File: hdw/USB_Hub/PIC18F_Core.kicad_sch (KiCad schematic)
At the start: 3 parts

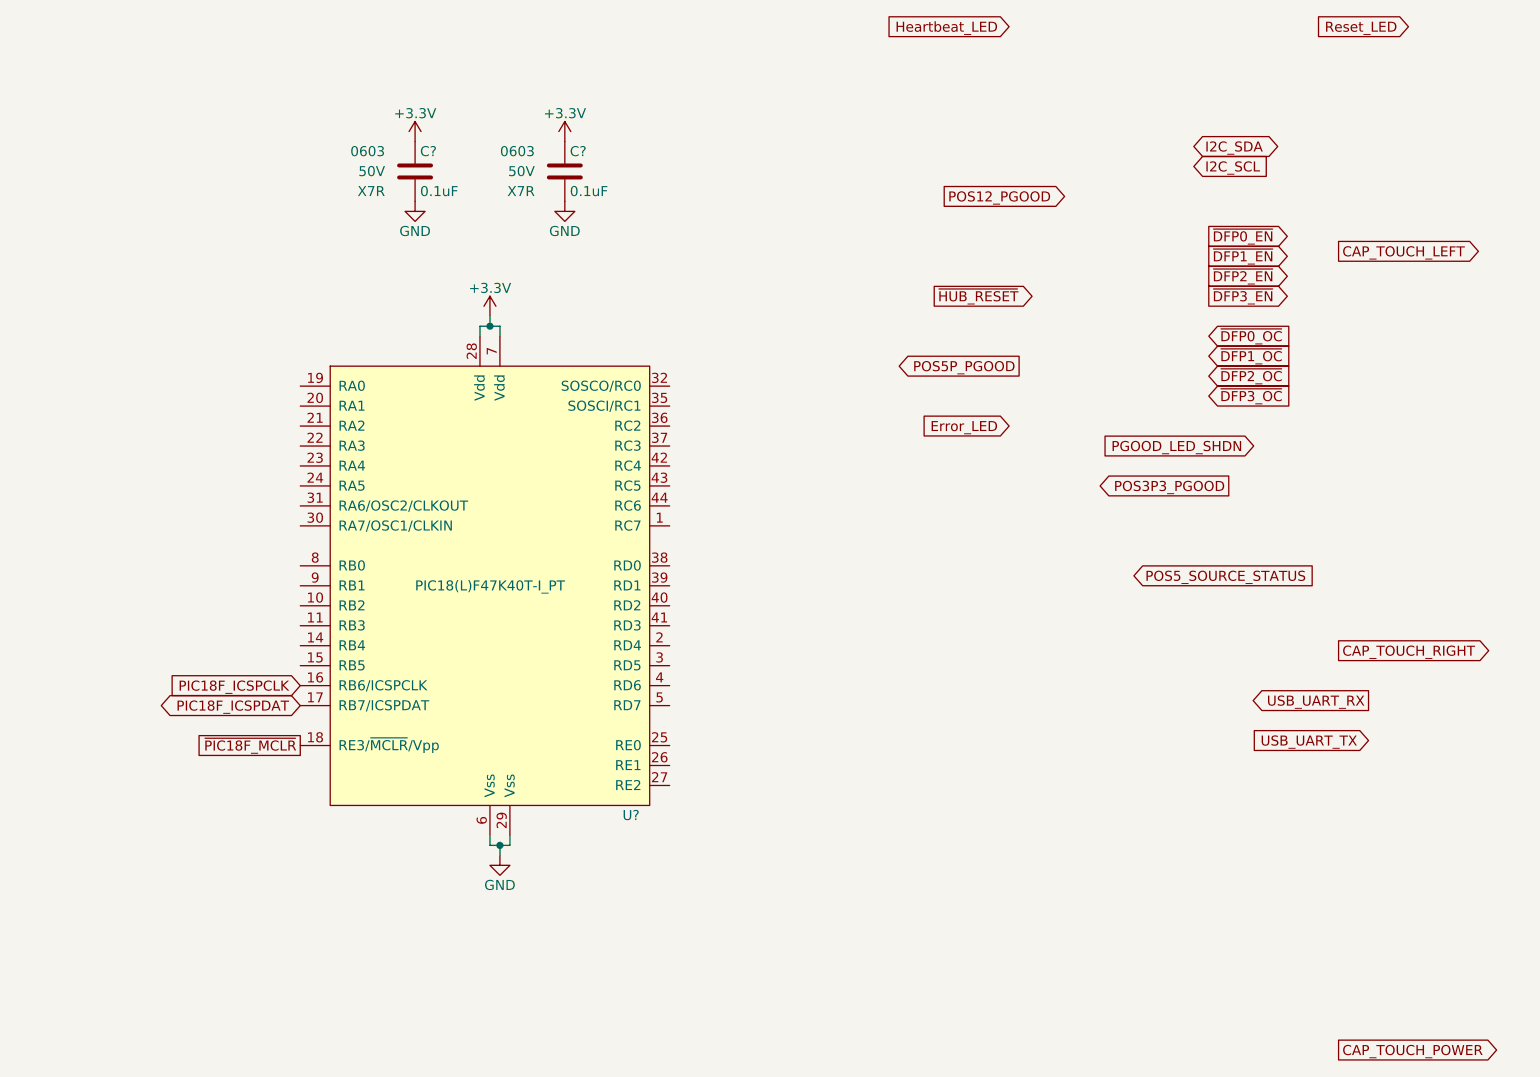
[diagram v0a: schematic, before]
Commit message: lots and lots of sch progress
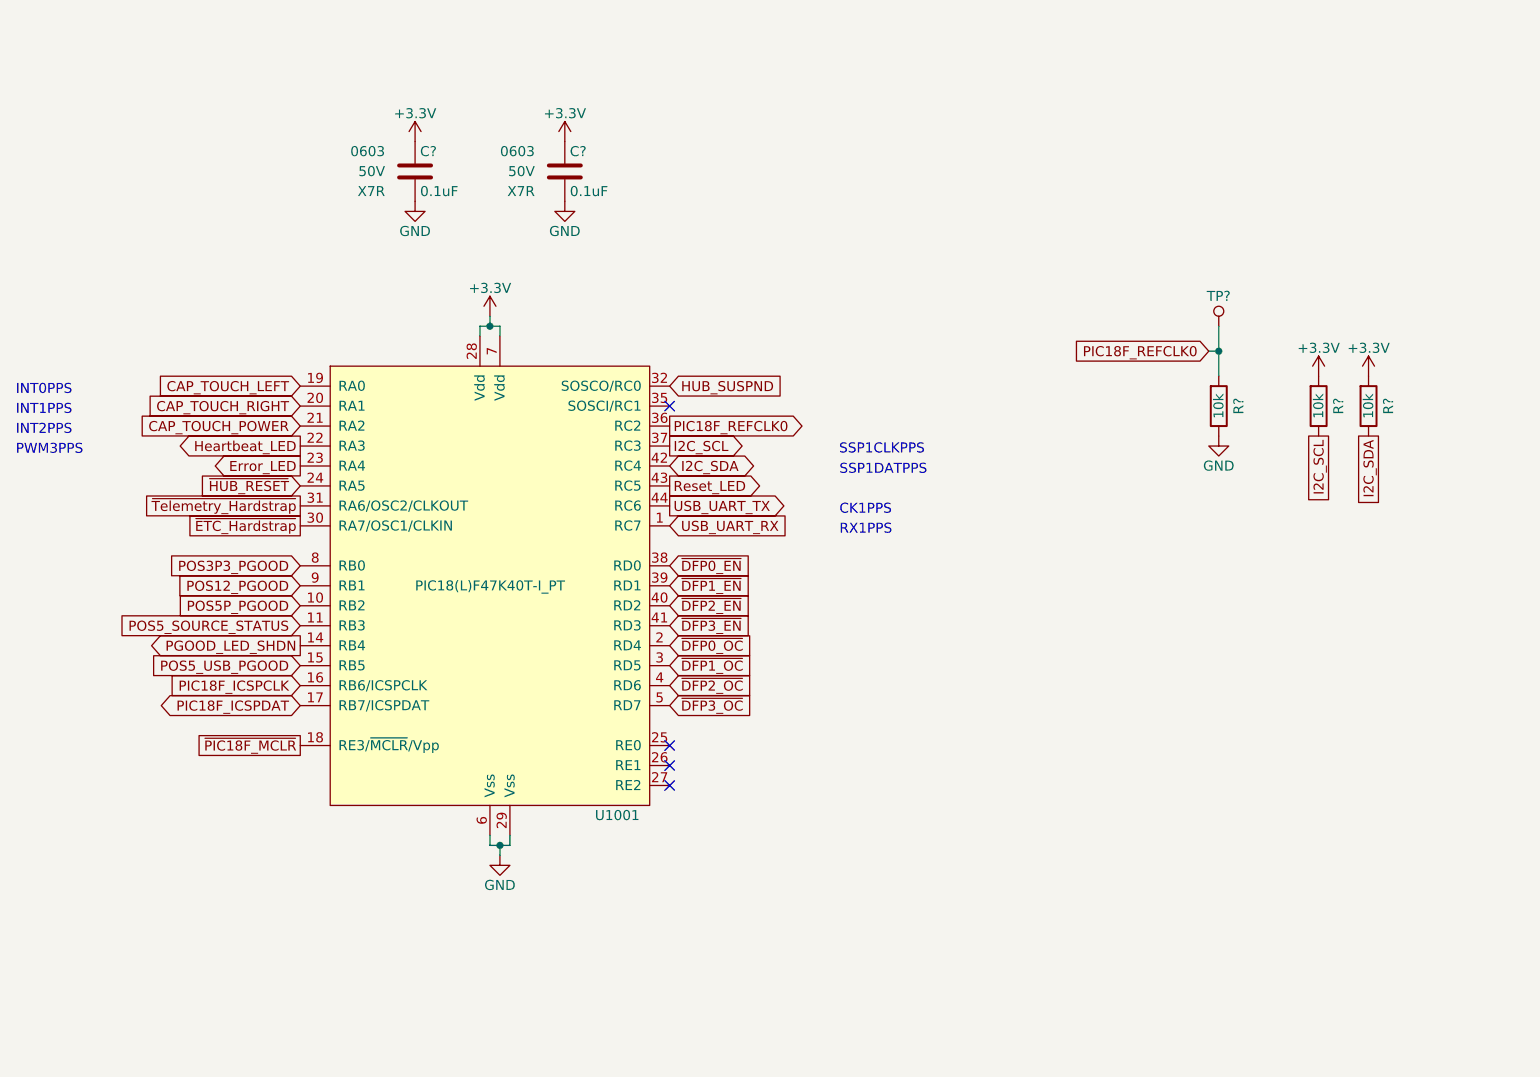
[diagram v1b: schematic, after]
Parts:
- added R? (x3): 10k, Resistors_SMD:R_0603, symbol Custom_Library:R_Custom
- added TP?: TP, Custom Footprints Library:Test_Point, symbol Custom_Library:TP
- gave numbers to parts that had none: 1
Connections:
- net +3.3V: now also R?.1, R?.1
- net CAP_TOUCH_LEFT: now also U1001.19 (RA0)
- net CAP_TOUCH_POWER: now also U1001.21 (RA2)
- net CAP_TOUCH_RIGHT: now also U1001.20 (RA1)
- net Error_LED: now also U1001.23 (RA4)
- net GND: now also R?.2
- net Heartbeat_LED: now also U1001.22 (RA3)
- net I2C_SCL: now also U1001.37 (RC3), R?.2
- net I2C_SDA: now also U1001.42 (RC4), R?.2
- net PGOOD_LED_SHDN: now also U1001.14 (RB4)
- net POS12_PGOOD: now also U1001.9 (RB1)
- net POS3P3_PGOOD: now also U1001.8 (RB0)
- net POS5P_PGOOD: now also U1001.10 (RB2)
- net POS5_SOURCE_STATUS: now also U1001.11 (RB3)
- net Reset_LED: now also U1001.43 (RC5)
- net USB_UART_RX: now also U1001.1 (RC7)
- net USB_UART_TX: now also U1001.44 (RC6)
- net ~{DFP0_EN}: now also U1001.38 (RD0)
- net ~{DFP0_OC}: now also U1001.2 (RD4)
- net ~{DFP1_EN}: now also U1001.39 (RD1)
- net ~{DFP1_OC}: now also U1001.3 (RD5)
- net ~{DFP2_EN}: now also U1001.40 (RD2)
- net ~{DFP2_OC}: now also U1001.4 (RD6)
- net ~{DFP3_EN}: now also U1001.41 (RD3)
- net ~{DFP3_OC}: now also U1001.5 (RD7)
- net ~{HUB_RESET}: now also U1001.24 (RA5)
- net POS5_USB_PGOOD: now reaches U1001.15 (RB5)
- net ~{ETC_Hardstrap}: now reaches U1001.30 (RA7/OSC1/CLKIN)
- net ~{Telemetry_Hardstrap}: now reaches U1001.31 (RA6/OSC2/CLKOUT)
- net HUB_SUSPND: now reaches U1001.32 (SOSCO/RC0)
- net PIC18F_REFCLK0: now reaches U1001.36 (RC2)
- net PIC18F_REFCLK0: now also R?.1, TP?.1 (TP)
- no-connect marks 0 -> 4
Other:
- note added: "CK1PPS"
- note added: "INT0PPS"
- note added: "INT1PPS"
- note added: "INT2PPS"
- note added: "PWM3PPS"
- note added: "RX1PPS"
- note added: "SSP1CLKPPS"
- note added: "SSP1DATPPS"

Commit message: pulled footprints into layout
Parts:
- R? (x3): Digi-Key PN YAG2321CT-ND -> (none)
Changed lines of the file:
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@@
       (effects (font (size 1.27 1.27)) (justify left) hide)
     )
-    (property "Digi-Key PN" "YAG2321CT-ND" (at 233.68 72.39 0)
+    (property "Digi-Key PN" "" (at 233.68 72.39 0)
       (effects (font (size 1.27 1.27)) hide)
     )
@@
       (effects (font (size 1.27 1.27)) (justify left) hide)
     )
-    (property "Digi-Key PN" "YAG2321CT-ND" (at 252.73 72.39 0)
+    (property "Digi-Key PN" "" (at 252.73 72.39 0)
       (effects (font (size 1.27 1.27)) hide)
     )
@@
       (effects (font (size 1.27 1.27)) (justify left) hide)
     )
-    (property "Digi-Key PN" "YAG2321CT-ND" (at 246.38 72.39 0)
-      (effects (font (size 1.27 1.27)) hide)
-    )
+    (property "Digi-Key PN" "" (at 246.38 72.39 0)
+      (effects (font (size 1.27 1.27)) hide)
+    )
